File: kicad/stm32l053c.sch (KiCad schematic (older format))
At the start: 29 parts, among them P1 SWD, P2 PWR, Q1 Q_PNP_BEC, SW1 SW_PUSH, SW2 SW_PUSH, SW3 SW_PUSH, U1 STM32L053C8_LQFP48, U2 TLV61225, Y1 Crystal

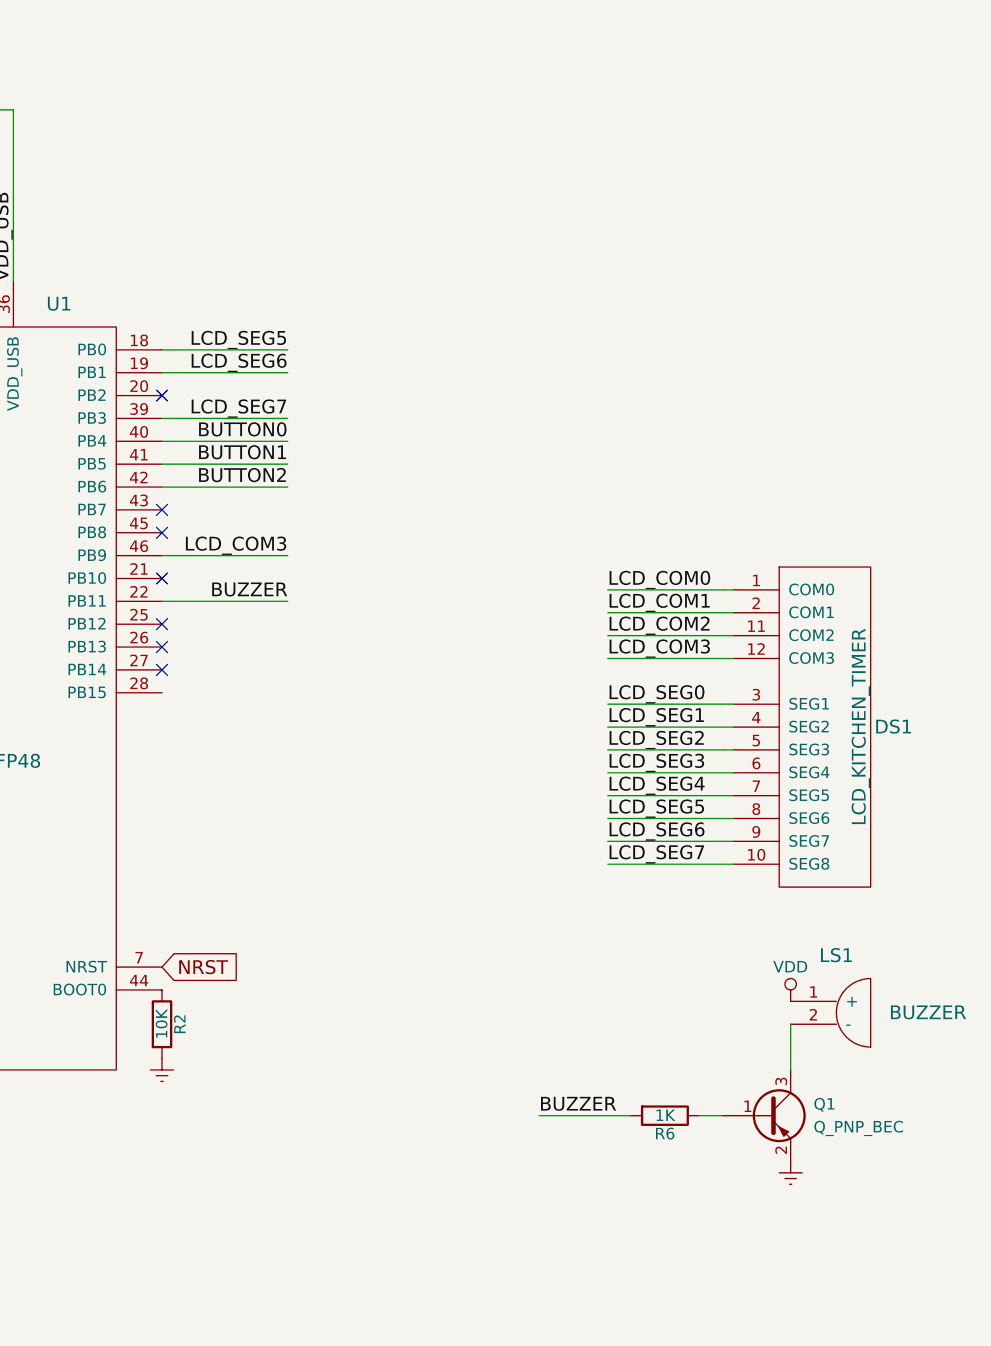
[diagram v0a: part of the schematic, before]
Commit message: STATE_RESET
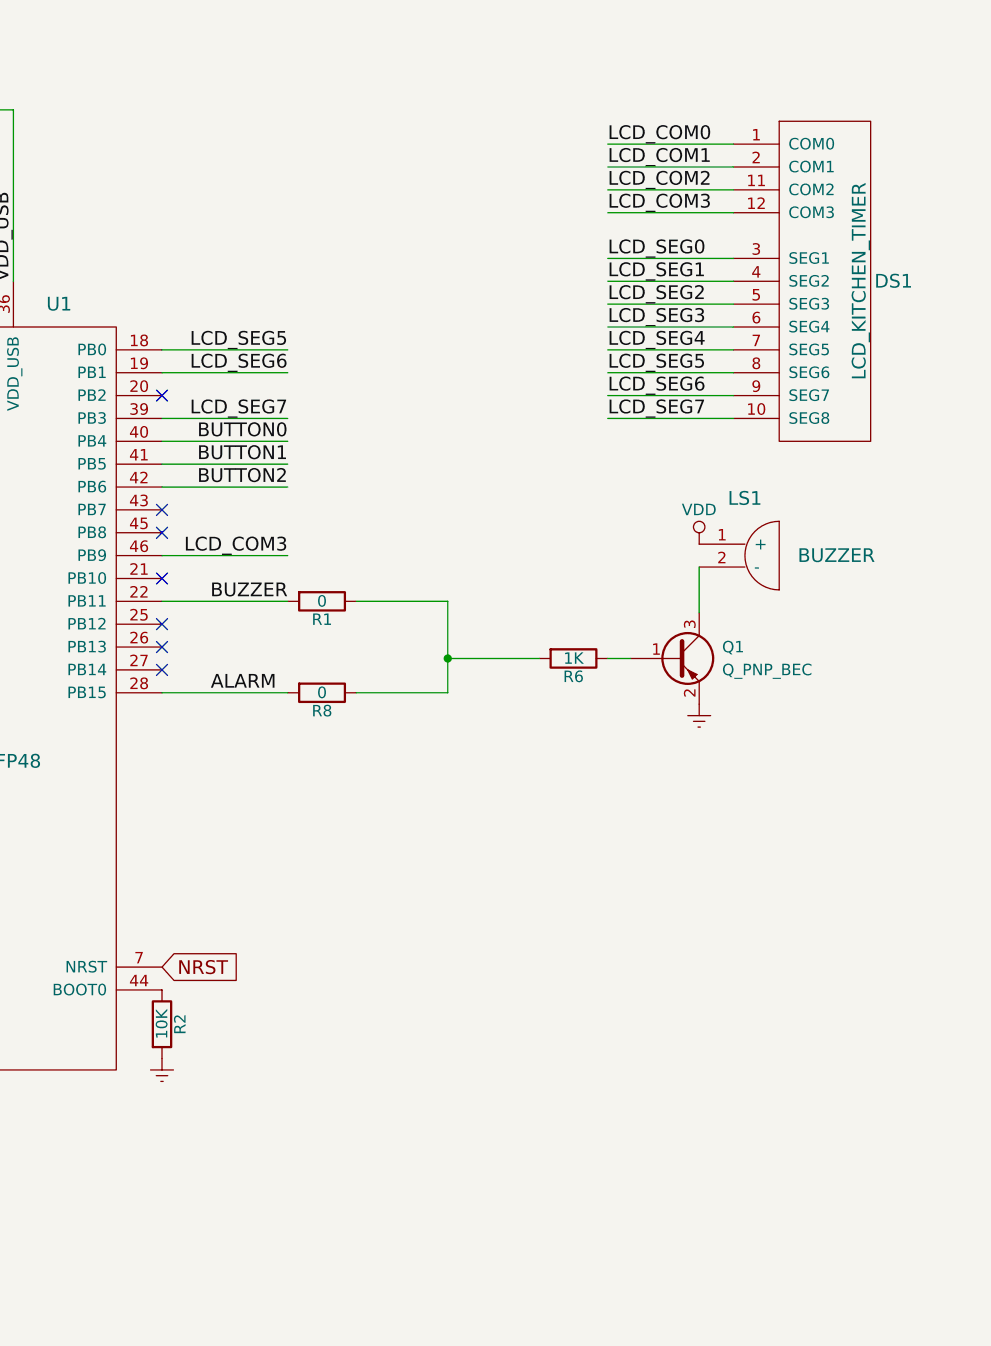
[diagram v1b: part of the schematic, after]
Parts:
- added R1, R8: 0, Resistors_SMD:R_0805_HandSoldering, symbol R
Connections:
- net BUZZER: now also R1.2; no longer R6.2
- net ALARM: now reaches U1.28 (PB15)
- net ALARM: now also R8.2
- new net: R1.1, R6.2, R8.1
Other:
- moved on the sheet: DS1, LS1, Q1, R6
